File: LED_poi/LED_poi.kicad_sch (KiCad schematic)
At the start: 44 parts, among them J1 Conn_01x03, J10 AVR-ICSP-TagConnect, J11 Ext_ACC, J12 RX, J13 TX, J2 Conn_01x03, J3 Conn_01x03, J4 D+, J5 Batt, J6 +5V, J7 KEY, J8 D-, J9 GND, Q1 2N7002, Q2 2N7002, Q3 2N7002, SW1 SW_Push, U1 ATmega32U4-A, U3 ADXL343, Y1 16MHz

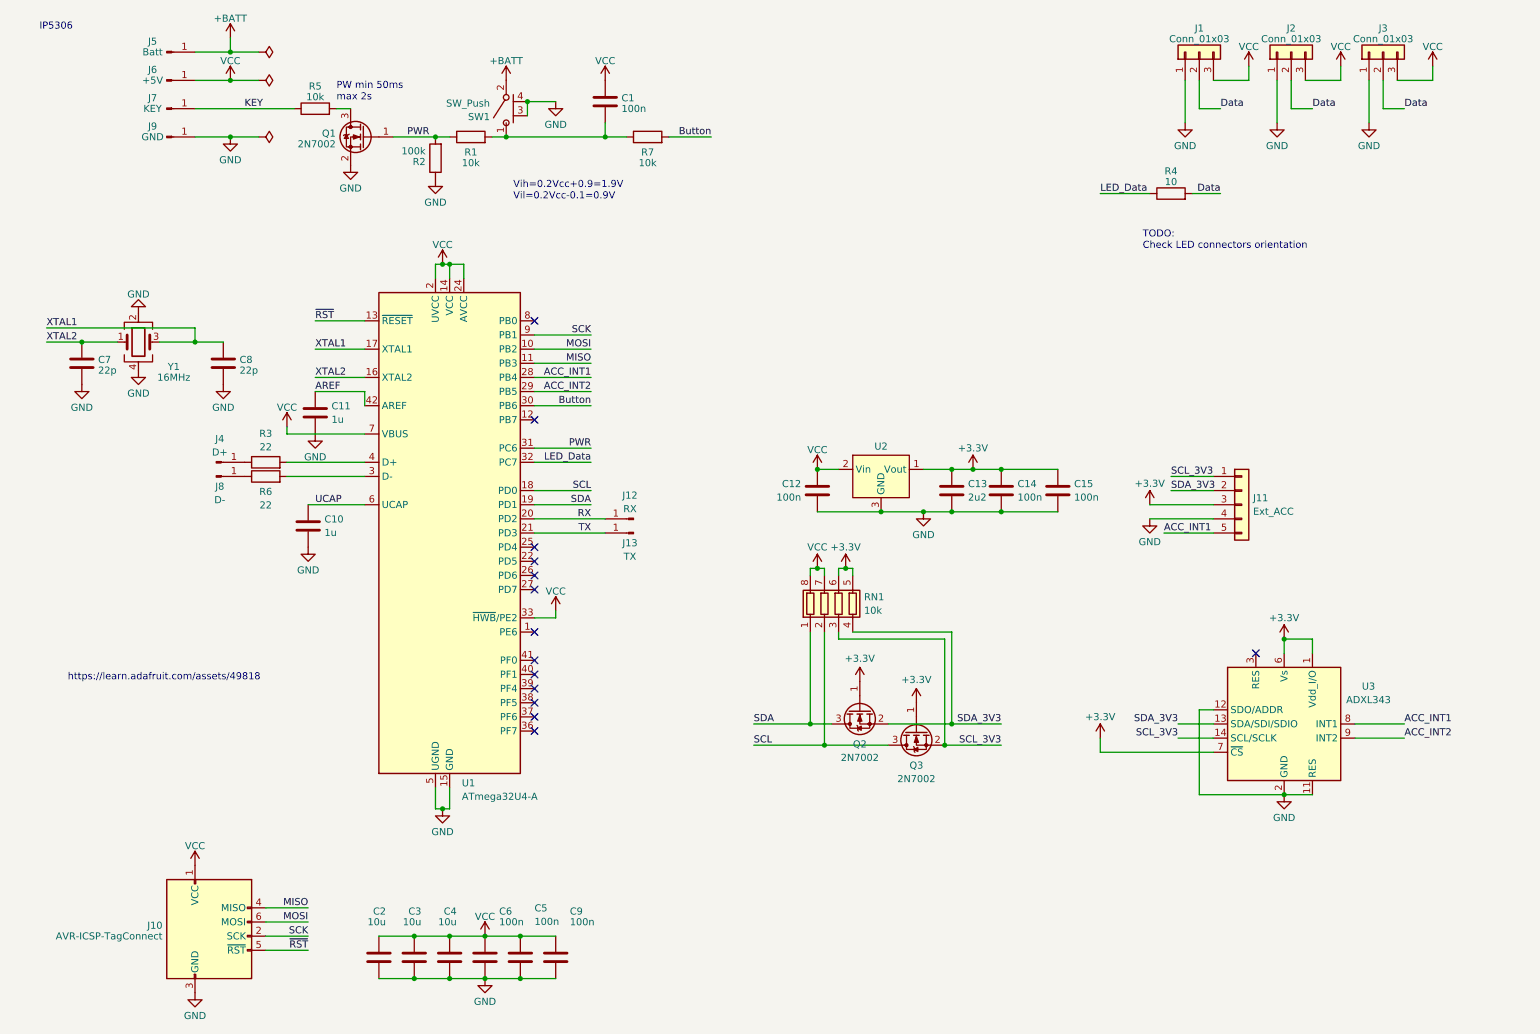
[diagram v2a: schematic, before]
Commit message: a
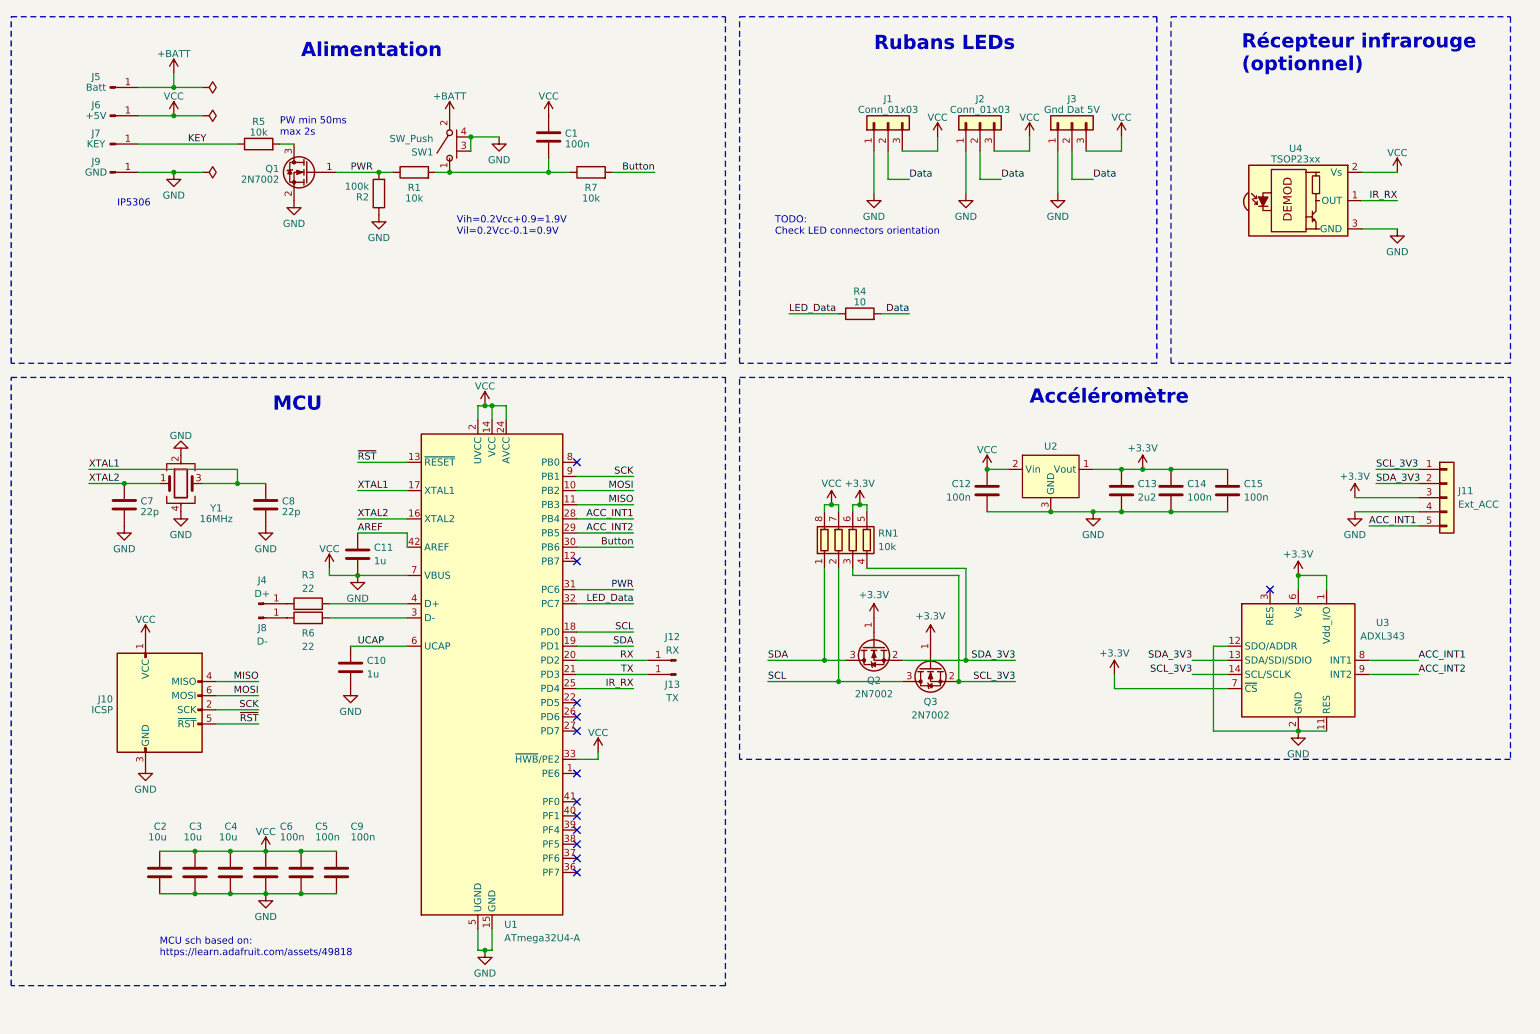
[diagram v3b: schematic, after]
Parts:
- added U4: TSOP23xx, OptoDevice:Vishay_MOLD-3Pin, symbol Interface_Optical:TSOP23xx
- J10: value AVR-ICSP-TagConnect -> ICSP
- J3: value Conn_01x03 -> Gnd Dat 5V
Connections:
- net VCC is gone; now on net GND: C1.2, C12.1, C2.1, C3.1, C4.1, C5.1, C6.1, C9.1, J1.3 (Pin_3), J10.1 (VCC), J2.3 (Pin_3), J3.3 (Pin_3), J6.1 (Pin_1), RN1.7 (R2.2), RN1.8 (R1.2), U1.14 (VCC), U1.2 (UVCC), U1.24 (AVCC), U1.33 (~{HWB}/PE2), U1.34 (VCC), U1.44 (AVCC), U1.7 (VBUS), U2.2 (Vin)
- net GND: now also U4.2 (Vs), U4.3 (GND)
- net IR_RX: now reaches U1.25 (PD4)
- net IR_RX: now also U4.1 (OUT)
- no-connect marks 14 -> 13
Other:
- note added: "Accéléromètre"
- note added: "Alimentation"
- note added: "MCU"
- note added: "MCU sch based on: https://learn.adafruit.com/assets/49818"
- note added: "Rubans LEDs"
- note added: "Récepteur infrarouge (optionnel)"
- note removed: "https://learn.adafruit.com/assets/49818"
- moved on the sheet: C1, C10, C11, C12, C13, C14, C15, C2, C3, C4, C5, C6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
